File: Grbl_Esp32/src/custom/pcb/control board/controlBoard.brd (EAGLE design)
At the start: 38 parts

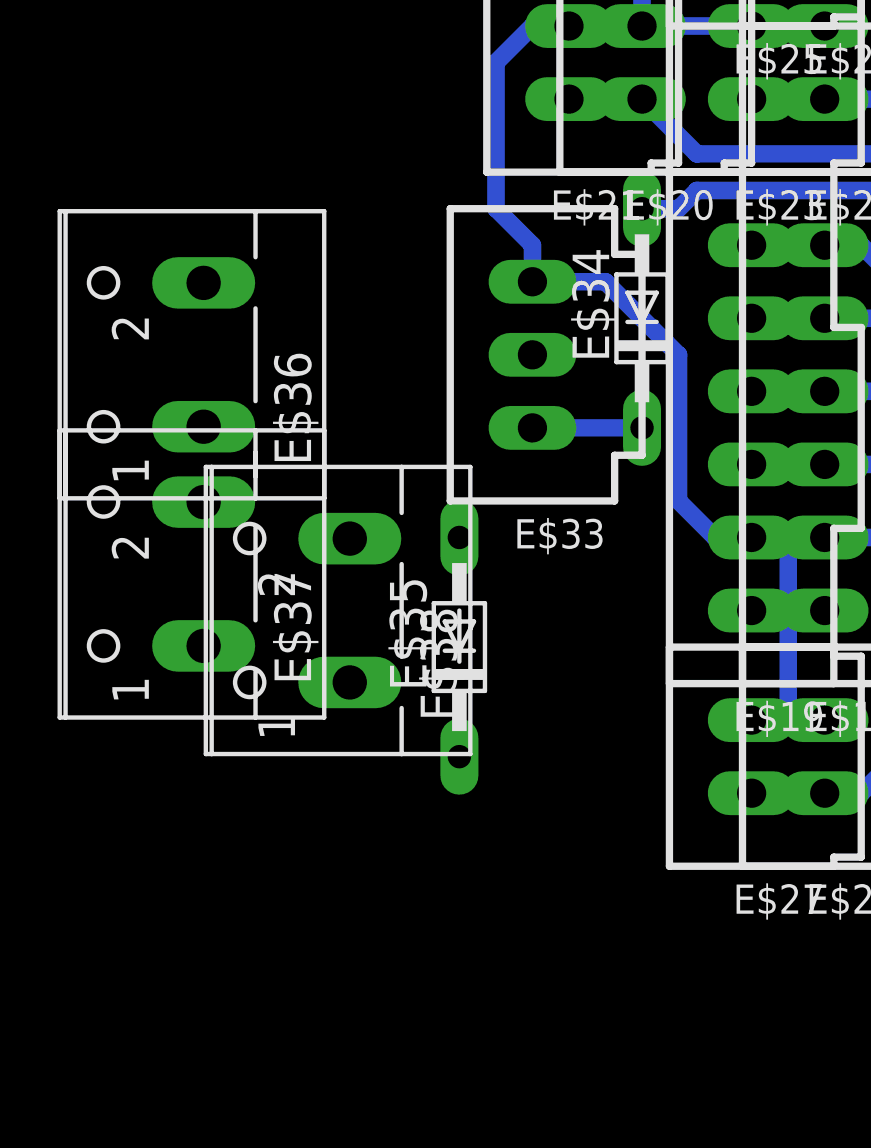
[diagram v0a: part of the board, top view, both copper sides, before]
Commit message: controlBoard
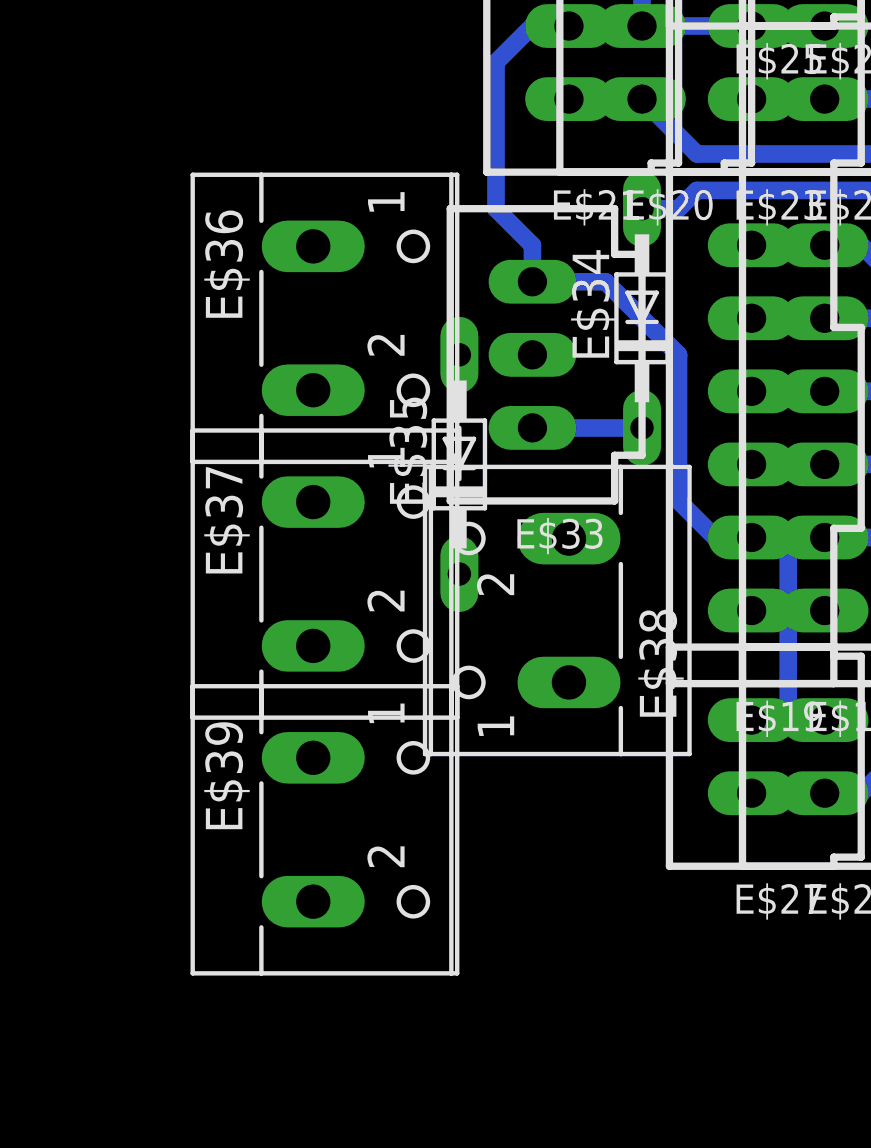
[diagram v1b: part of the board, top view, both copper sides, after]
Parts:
- added E$39: (no value), con-wago-500:W237-102
- moved E$38 7.62 mm to (8.89, 40.6)
- moved E$36 6.48 mm to (2.54, 50.8), turned to 270 degrees
- moved E$35 6.35 mm to (6.35, 45.7)
- moved E$37 6.35 mm to (2.54, 41.9), turned to 270 degrees
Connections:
- new net S$13: E$33.2, E$35.A, E$38.2
- new net S$14: E$35.C, E$38.1
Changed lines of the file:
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@@
 <attribute name="VALUE" x="15.113" y="49.276" size="1.27" layer="27" ratio="10" rot="R90"/>
 </element>
-<element name="E$35" library="diode" library_urn="urn:adsk.eagle:library:210" package="DO34-7" package3d_urn="urn:adsk.eagle:package:43348/1" value="" x="6.35" y="39.37" rot="R90">
-<attribute name="NAME" x="5.207" y="37.846" size="1.27" layer="25" ratio="10" rot="R90"/>
-<attribute name="VALUE" x="8.763" y="37.846" size="1.27" layer="27" ratio="10" rot="R90"/>
-</element>
-<element name="E$36" library="con-wago-500" library_urn="urn:adsk.eagle:library:195" package="W237-102" package3d_urn="urn:adsk.eagle:package:10688/1" value="" x="-3.81" y="49.53" rot="R90">
-<attribute name="NAME" x="1.1938" y="45.6838" size="1.27" layer="25" ratio="10" rot="R90"/>
-<attribute name="VALUE" x="3.81" y="44.49" size="1.27" layer="27" ratio="10" rot="R90"/>
-</element>
-<element name="E$37" library="con-wago-500" library_urn="urn:adsk.eagle:library:195" package="W237-102" package3d_urn="urn:adsk.eagle:package:10688/1" value="" x="-3.81" y="41.91" rot="R90">
-<attribute name="NAME" x="1.1938" y="38.0638" size="1.27" layer="25" ratio="10" rot="R90"/>
-<attribute name="VALUE" x="3.81" y="36.87" size="1.27" layer="27" ratio="10" rot="R90"/>
-</element>
-<element name="E$38" library="con-wago-500" library_urn="urn:adsk.eagle:library:195" package="W237-102" package3d_urn="urn:adsk.eagle:package:10688/1" value="" x="1.27" y="40.64" rot="R90">
-<attribute name="NAME" x="6.2738" y="36.7938" size="1.27" layer="25" ratio="10" rot="R90"/>
-<attribute name="VALUE" x="8.89" y="35.6" size="1.27" layer="27" ratio="10" rot="R90"/>
+<element name="E$35" library="diode" library_urn="urn:adsk.eagle:library:210" package="DO34-7" package3d_urn="urn:adsk.eagle:package:43348/1" value="" x="6.35" y="45.72" rot="R90">
+<attribute name="NAME" x="5.207" y="44.196" size="1.27" layer="25" ratio="10" rot="R90"/>
+<attribute name="VALUE" x="8.763" y="44.196" size="1.27" layer="27" ratio="10" rot="R90"/>
+</element>
+<element name="E$36" library="con-wago-500" library_urn="urn:adsk.eagle:library:195" package="W237-102" package3d_urn="urn:adsk.eagle:package:10688/1" value="" x="2.54" y="50.8" rot="R270">
+<attribute name="NAME" x="-2.4638" y="54.6462" size="1.27" layer="25" ratio="10" rot="R270"/>
+<attribute name="VALUE" x="-5.08" y="55.84" size="1.27" layer="27" ratio="10" rot="R270"/>
+</element>
+<element name="E$37" library="con-wago-500" library_urn="urn:adsk.eagle:library:195" package="W237-102" package3d_urn="urn:adsk.eagle:package:10688/1" value="" x="2.54" y="41.91" rot="R270">
+<attribute name="NAME" x="-2.4638" y="45.7562" size="1.27" layer="25" ratio="10" rot="R270"/>
+<attribute name="VALUE" x="-5.08" y="46.95" size="1.27" layer="27" ratio="10" rot="R270"/>
+</element>
+<element name="E$38" library="con-wago-500" library_urn="urn:adsk.eagle:library:195" package="W237-102" package3d_urn="urn:adsk.eagle:package:10688/1" value="" x="8.89" y="40.64" rot="R90">
+<attribute name="NAME" x="13.8938" y="36.7938" size="1.27" layer="25" ratio="10" rot="R90"/>
+<attribute name="VALUE" x="16.51" y="35.6" size="1.27" layer="27" ratio="10" rot="R90"/>
+</element>
+<element name="E$39" library="con-wago-500" library_urn="urn:adsk.eagle:library:195" package="W237-102" package3d_urn="urn:adsk.eagle:package:10688/1" value="" x="2.54" y="33.02" rot="R270">
+<attribute name="NAME" x="-2.4638" y="36.8662" size="1.27" layer="25" ratio="10" rot="R270"/>
+<attribute name="VALUE" x="-5.08" y="38.06" size="1.27" layer="27" ratio="10" rot="R270"/>
 </element>
 </elements>
@@
 <wire x1="19.05" y1="53.34" x2="16.51" y2="53.34" width="0.6096" layer="16"/>
 </signal>
+<signal name="S$13">
+<contactref element="E$35" pad="A"/>
+<contactref element="E$33" pad="2"/>
+<wire x1="8.89" y1="49.53" x2="6.35" y2="49.53" width="0" layer="19" extent="1-16"/>
+<contactref element="E$38" pad="2"/>
+<wire x1="10.16" y1="43.14" x2="6.35" y2="49.53" width="0" layer="19" extent="1-16"/>
+</signal>
+<signal name="S$14">
+<contactref element="E$38" pad="1"/>
+<contactref element="E$35" pad="C"/>
+<wire x1="6.35" y1="41.91" x2="10.16" y2="38.14" width="0" layer="19" extent="1-16"/>
+</signal>
 </signals>
